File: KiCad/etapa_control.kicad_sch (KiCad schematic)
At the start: 26 parts, among them J1 DE9_Pins, J2 DE9_Pins, J3 Conn_01x05, SW3 SW_Push_Dual, U20 PIC24HJ128GP502, U3 SN65HVD230, U4 MAX3232, Y1 Crystal

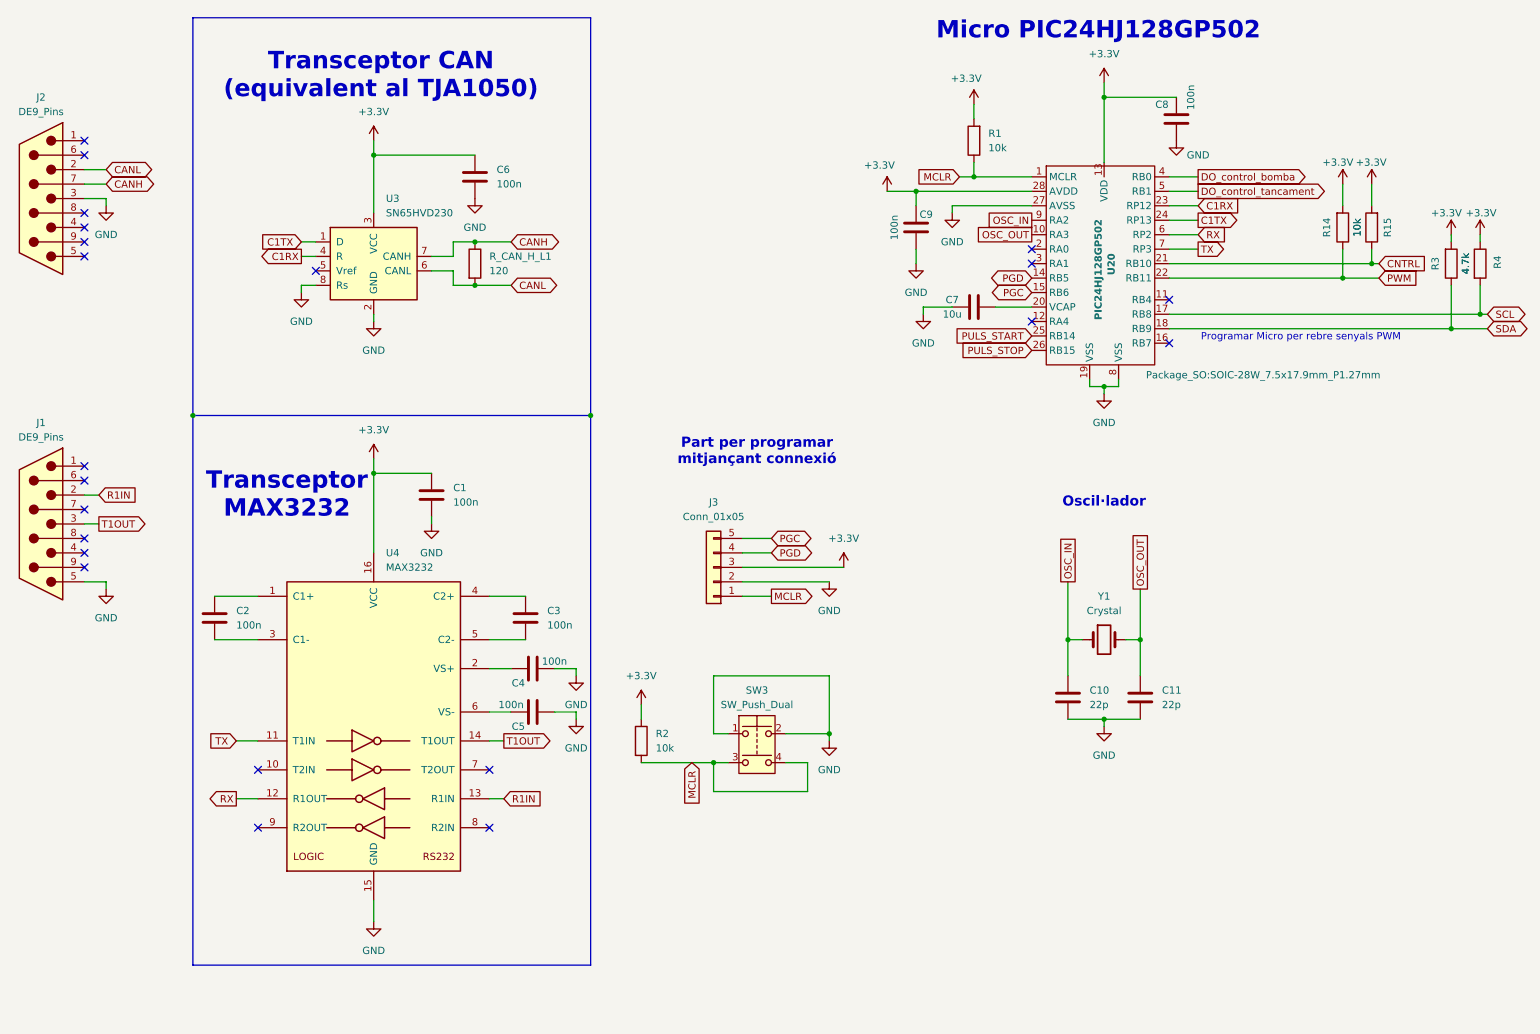
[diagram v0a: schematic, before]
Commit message: Correccions dels sheets i títols fetes
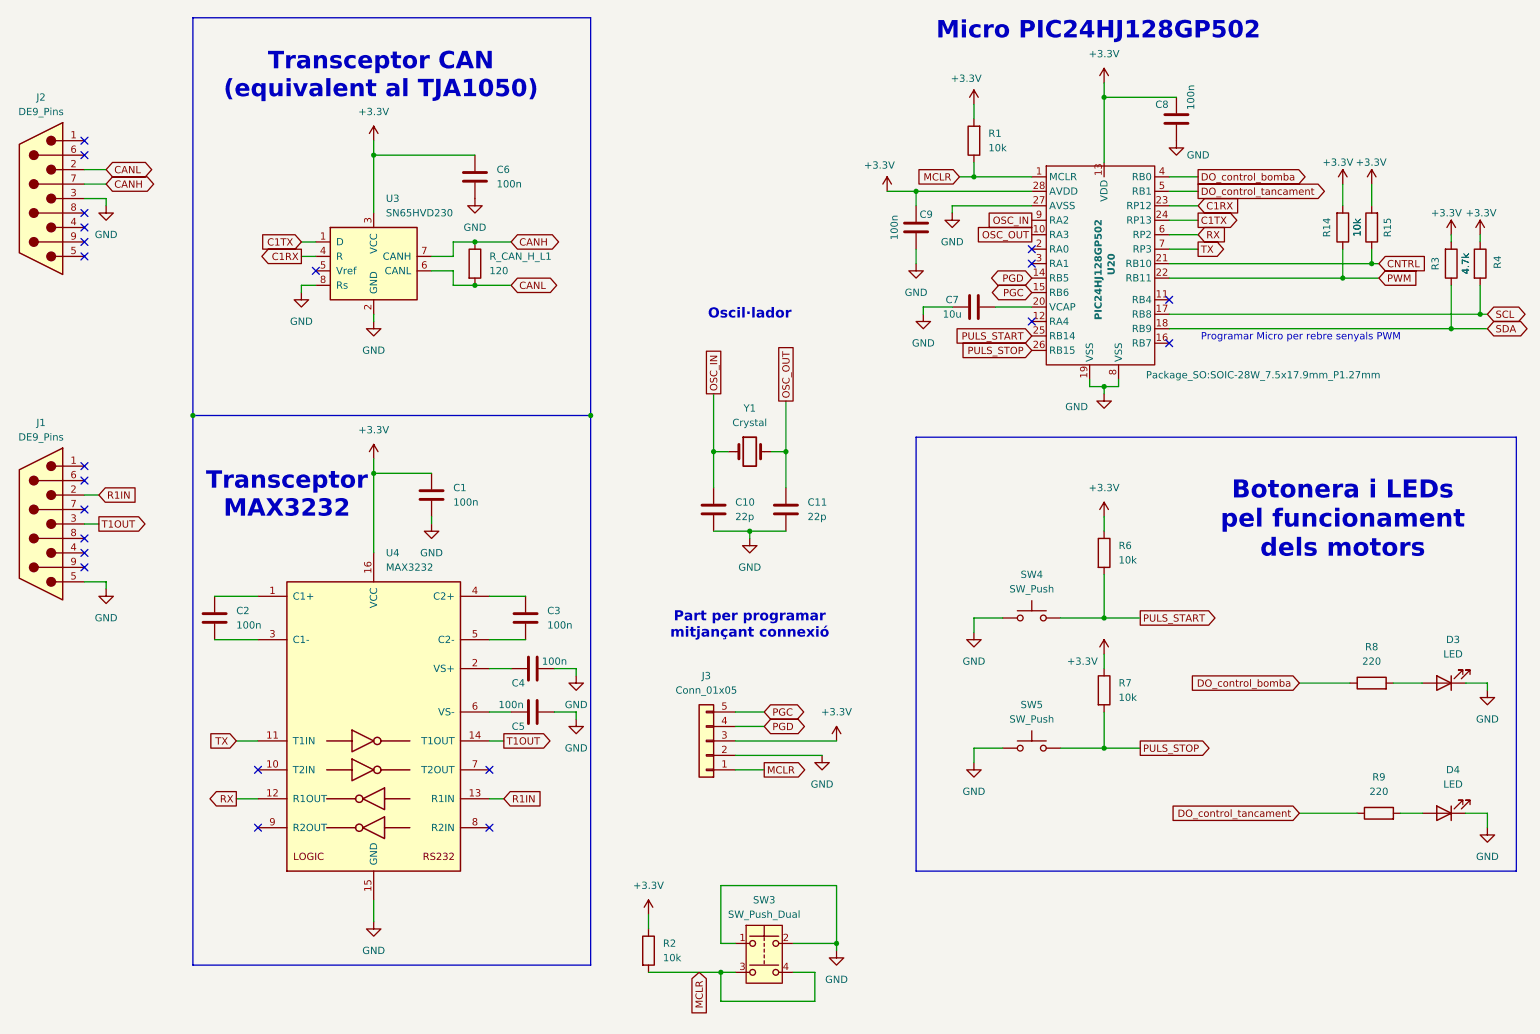
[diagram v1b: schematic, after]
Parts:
- added D3, D4: LED, LED_THT:LED_D3.0mm, symbol Device:LED
- added R6, R7: 10k, Resistor_SMD:R_0805_2012Metric, symbol Device:R
- added R8, R9: 220, Resistor_SMD:R_0805_2012Metric, symbol Device:R
- added SW4, SW5: SW_Push, Button_Switch_SMD:SW_DIP_SPSTx01_Slide_Copal_CHS-01B_W7.62mm_P1.27mm, symbol Switch:SW_Push
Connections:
- net +3.3V: now also R6.1, R7.1
- net DO_control_bomba: now also R8.1
- net DO_control_tancament: now also R9.1
- net GND: now also D3.1 (K), D4.1 (K), SW4.1, SW5.1
- net PULS_START: now also R6.2, SW4.2
- net PULS_STOP: now also R7.2, SW5.2
- new net: D4.2 (A), R9.2
- new net: D3.2 (A), R8.2
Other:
- note added: "Botonera i LEDs pel funcionament dels motors"
- moved on the sheet: C10, C11, J3, R2, SW3, Y1
